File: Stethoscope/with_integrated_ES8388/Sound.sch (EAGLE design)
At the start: 52 parts, among them IC1 ES8388, IC2 TLV9002IDDFR, J1 SJ-3523-SMT-TR, J3 SJ2-3574A-SMT-TR

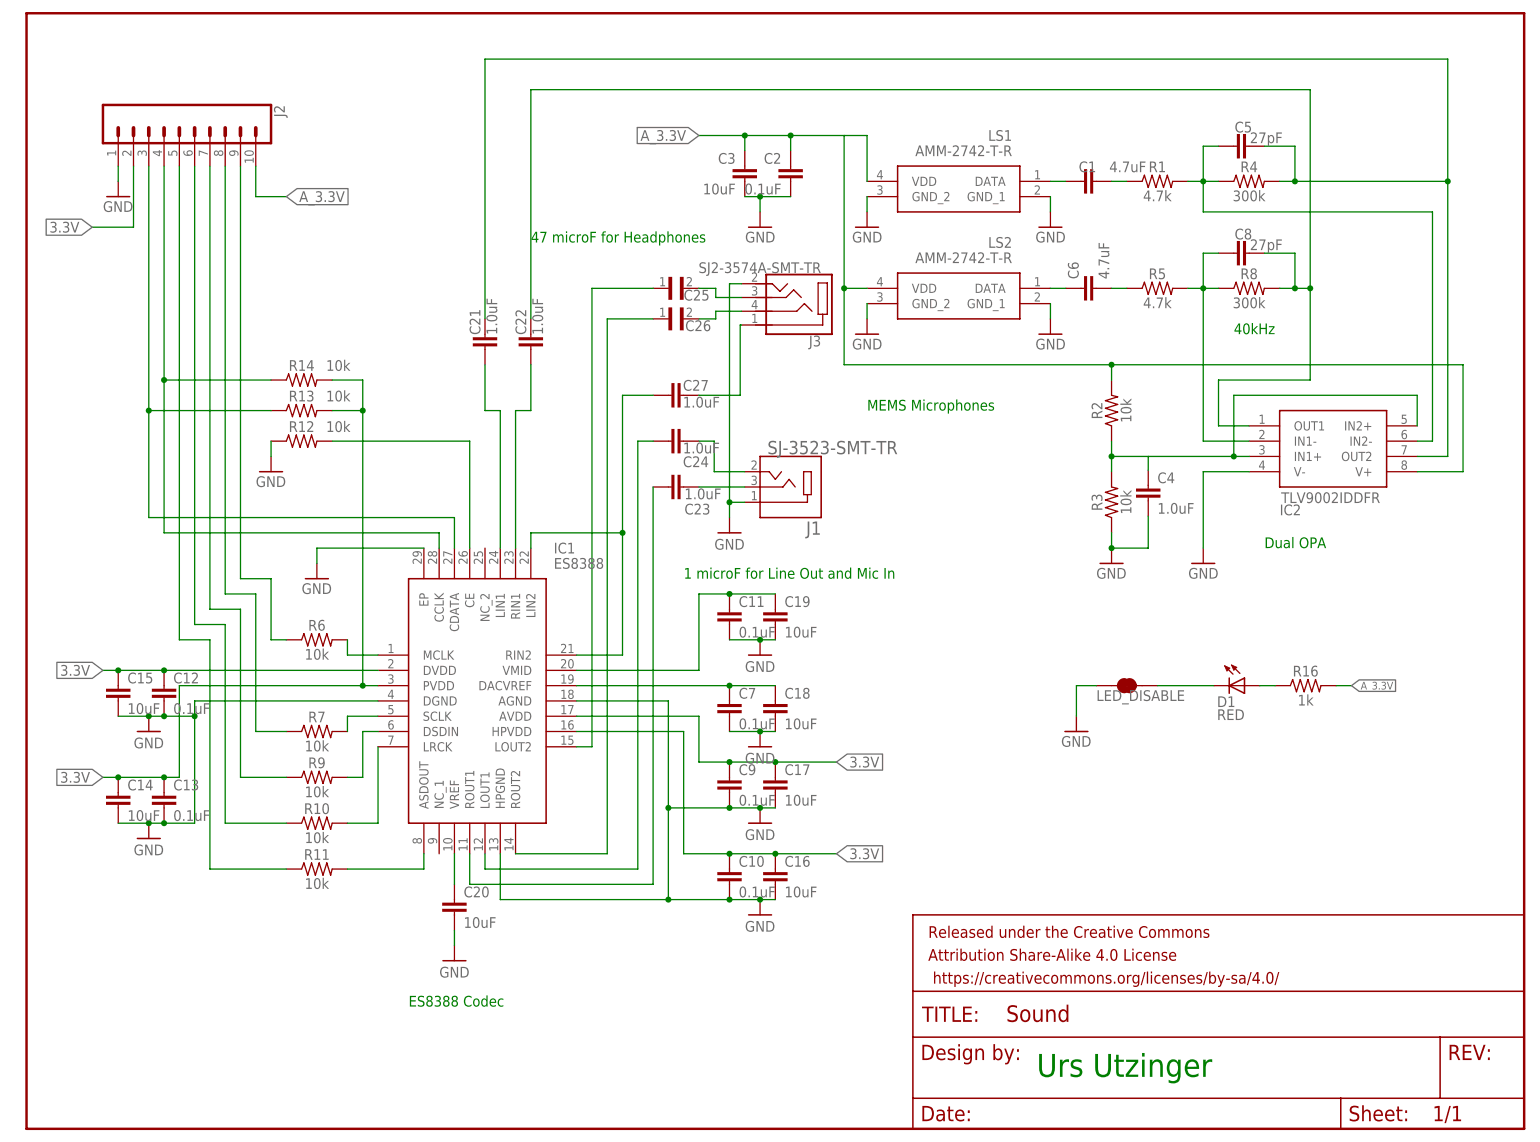
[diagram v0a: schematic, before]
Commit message: Sound Board Updates
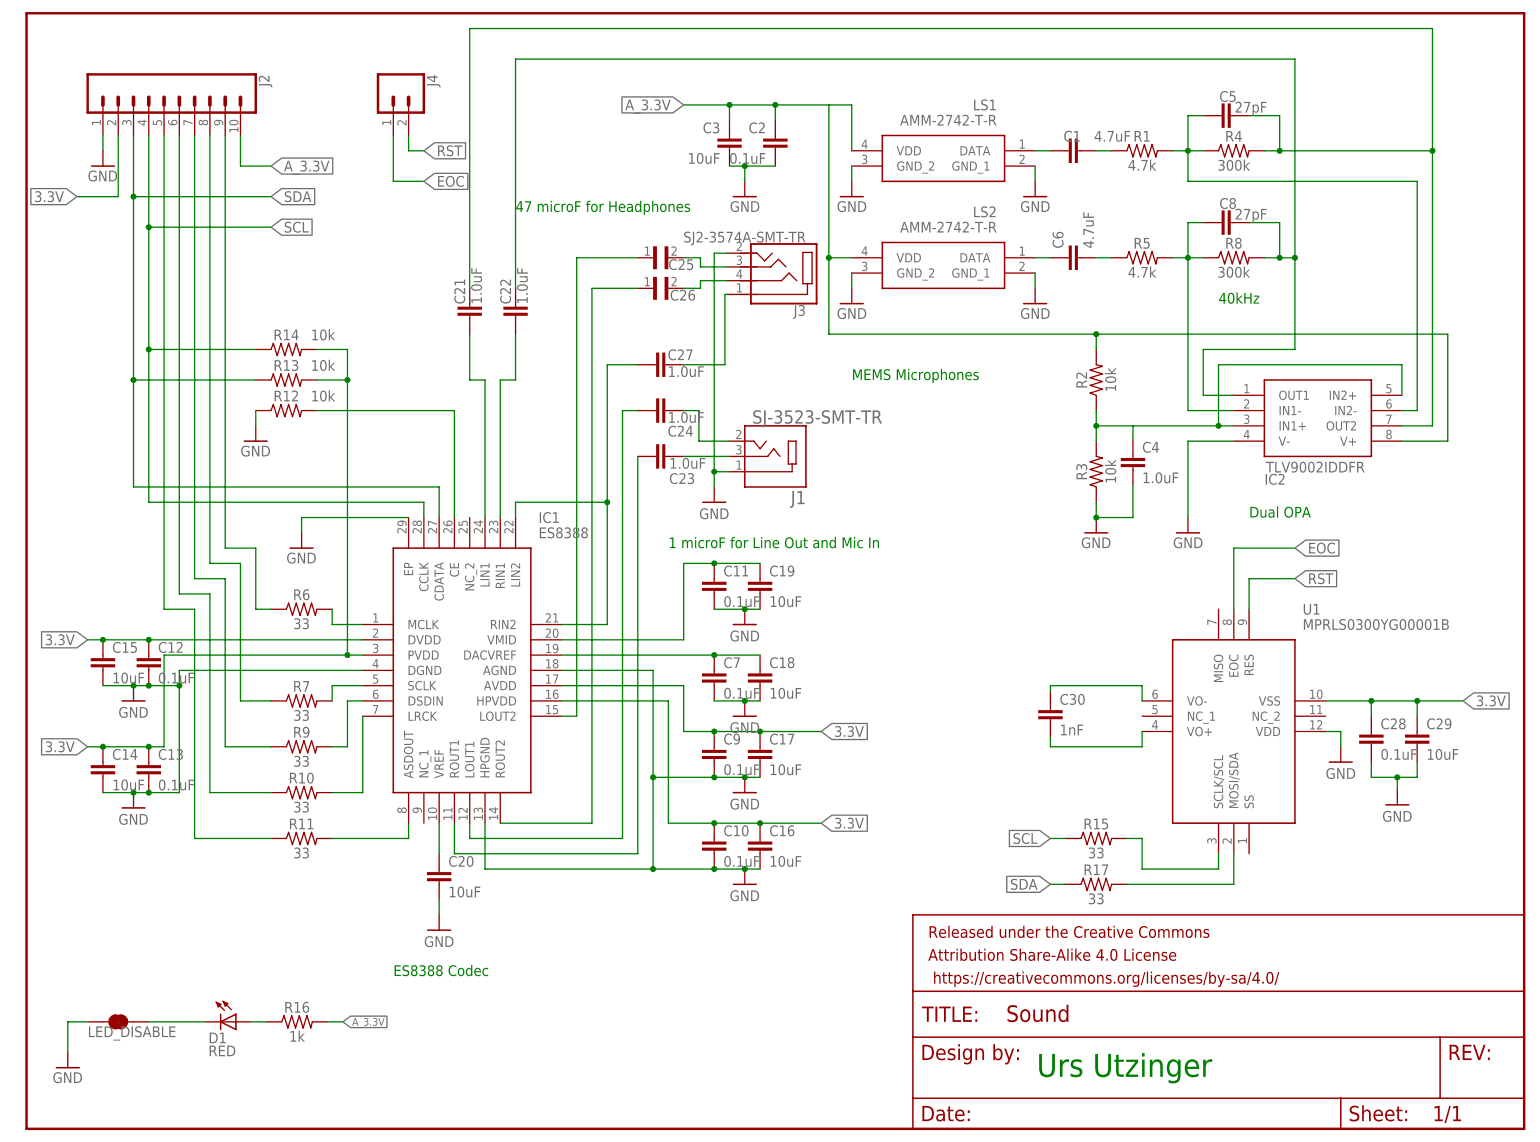
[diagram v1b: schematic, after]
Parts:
- added C28: 0.1uF, SparkFun-Capacitors:0.1UF-0603-25V-5%
- added C29: 10uF, SparkFun-Capacitors:10UF-0603-6.3V-20%
- added C30: 1nF, SparkFun-Capacitors:1.0NF/1000PF-0603-50V-10%
- added J4: (no value), SparkFun-Connectors:CONN_02
- added R15, R17: 33, SparkFun-Resistors:33OHM-0603-1/10W-1%
- added U1: MPRLS0300YG00001B, MPRLS0300YG00001B:MPRLS0300YG00001B
- C1, C6: device SparkFun-Capacitors:4.7UF0603 -> SparkFun-Capacitors:4.7UF-0603-6.3V-(10%)
- R10, R11, R6, R7, R9: value 10k -> 33; device SparkFun-Resistors:10KOHM-0603-1/10W-1% -> SparkFun-Resistors:33OHM-0603-1/10W-1%
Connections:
- new net EOC: J4.1, U1.EOC
- new net N$11: C30.2, U1.VO+
- new net N$6: R17.2, U1.MOSI/SDA
- new net N$7: R15.2, U1.SCLK/SCL
- new net N$9: C30.1, U1.VO-
- new net RST: J4.2, U1.RES
- net 3.3V: now also C28.1, C29.1, U1.VSS
- net GND: now also C28.2, C29.2, U1.VDD
- net SCL: now also R15.1
- net SDA: now also R17.1
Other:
- moved on the sheet: C1, C10, C11, C12, C13, C14, C15, C16, C17, C18, C19, C2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
